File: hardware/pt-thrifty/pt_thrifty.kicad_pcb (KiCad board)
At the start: 2 copper layers, 25.4 x 31.6 mm, 23 parts, among them J1 Conn_01x09, J2 Conn_01x09, J3 SJ-43514-SMT-TR, SW1 PTS636 SM50J SMTR LFS, SW2 SW_Push_Shielded, U2 MCP6273T-E/CH

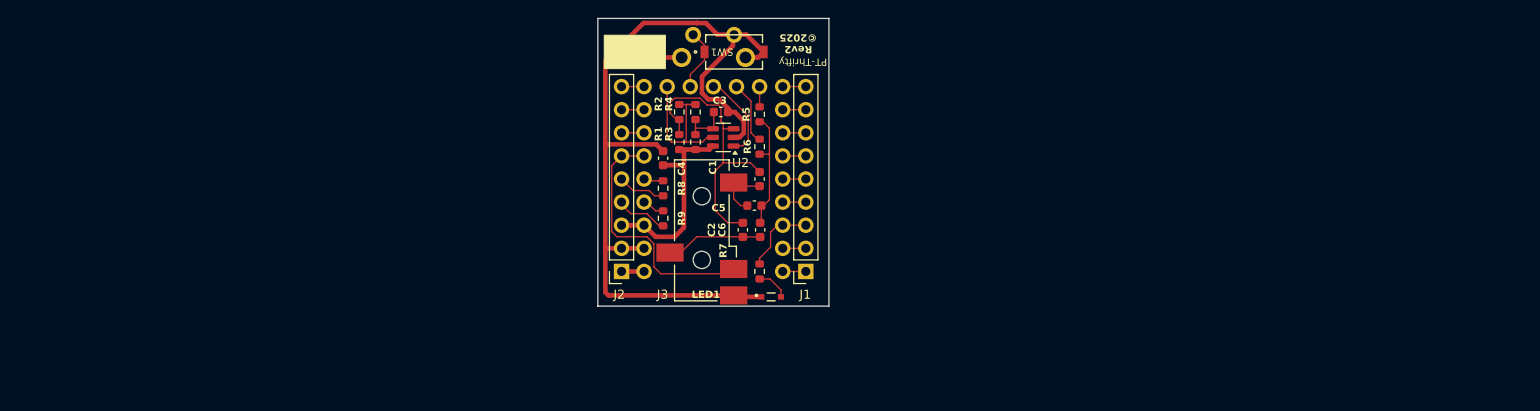
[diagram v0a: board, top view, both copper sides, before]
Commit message: WIP pt-thrifty rev3 sch/pcb
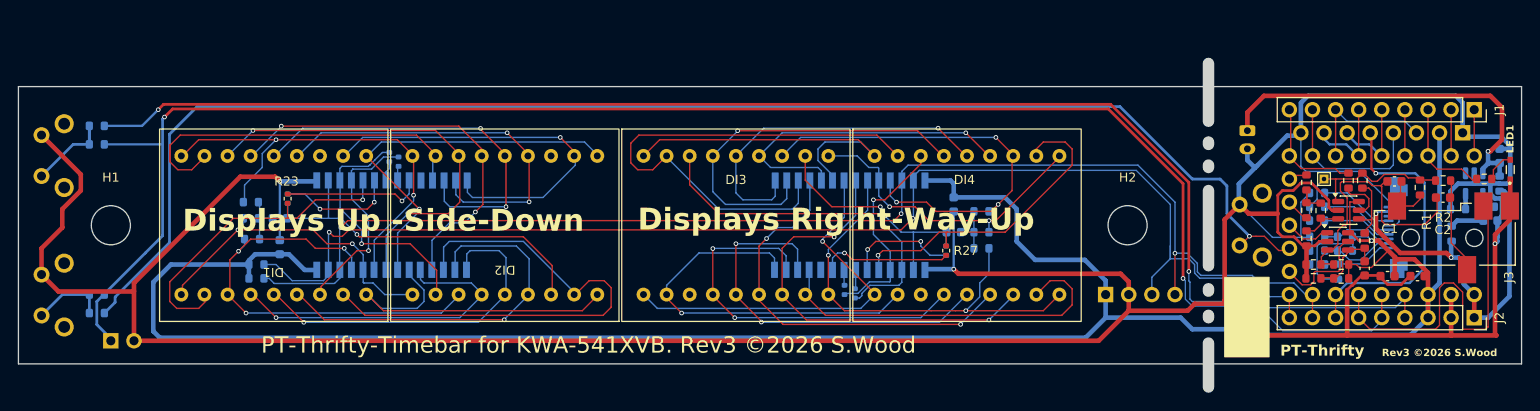
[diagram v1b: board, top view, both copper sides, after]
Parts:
- removed C6: 100nF, Capacitor_SMD:C_0603_1608Metric
- added C7: 10uF, Capacitor_SMD:C_0603_1608Metric, B.Cu at (166.3, 89.2)
- added C8: 10uF, Capacitor_SMD:C_0603_1608Metric, B.Cu at (92.2, 93.9)
- added C81: 1uF, Capacitor_SMD:C_0603_1608Metric, B.Cu at (225.3, 90.9)
- added C82: 1uF, Capacitor_SMD:C_0603_1608Metric, B.Cu at (226.3, 83.8)
- added D1: D, Diode_SMD:D_0603_1608Metric, B.Cu at (166.3, 92.2)
- added D2: D, Diode_SMD:D_0603_1608Metric, B.Cu at (92.2, 90.7)
- added DI1: KWA-541XVB, Displays:KWA-541XVB, F.Cu at (91.6, 91.4)
- added DI2: KWA-541XVB, Displays:KWA-541XVB, F.Cu at (117.0, 91.4)
- added DI3: KWA-541XVB, Displays:KWA-541XVB, F.Cu at (142.4, 91.4)
- added DI4: KWA-541XVB, Displays:KWA-541XVB, F.Cu at (167.8, 91.4)
- added H1: MountingHole, MountingHole:MountingHole_4.3mm_M4, F.Cu at (73.7, 91.4)
- added H2: MountingHole, MountingHole:MountingHole_4.3mm_M4, F.Cu at (185.4, 91.4)
- added J4: Conn_01x08, Connector_PinSocket_2.54mm:PinSocket_1x08_P2.54mm_Vertical, B.Cu at (222.2, 81.3)
- added J5: Conn_01x04, Connector_PinSocket_2.54mm:PinSocket_1x04_P2.54mm_Vertical, B.Cu at (183.0, 99.1)
- added J6: Conn_01x02, Connector_PinSocket_2.54mm:PinSocket_1x02_P2.54mm_Vertical, B.Cu at (73.7, 104.1)
- added J81: Conn_01x02, Connector_JST:JST_PH_B2B-PH-K_1x02_P2.00mm_Vertical, B.Cu at (198.6, 81.0)
- added J99: Conn_01x10, Connector_FFC-FPC:Amphenol_F32Q-1A7x1-11010_1x10-1MP_P0.5mm_Horizontal, B.Cu at (217.0, 91.7)
- added R10: 100K, Resistor_SMD:R_0603_1608Metric, F.Cu at (206.7, 89.8)
- added R11: 100K, Resistor_SMD:R_0603_1608Metric, F.Cu at (205.1, 92.9)
- added R12: 100K, Resistor_SMD:R_0603_1608Metric, F.Cu at (211.5, 93.1)
- added R13: 100K, Resistor_SMD:R_0603_1608Metric, F.Cu at (211.2, 86.5)
- added R14: 100R, Resistor_SMD:R_0603_1608Metric, F.Cu at (209.7, 86.5)
- added R15: 0R, Resistor_SMD:R_0603_1608Metric, B.Cu at (72.1, 101.1)
- added R16: 0R, Resistor_SMD:R_0603_1608Metric, B.Cu at (72.1, 99.1)
- added R17: 0R, Resistor_SMD:R_0603_1608Metric, B.Cu at (72.1, 80.5)
- added R18: 0R, Resistor_SMD:R_0603_1608Metric, B.Cu at (72.1, 82.5)
- added R20: 0R, Resistor_SMD:R_0402_1005Metric, B.Cu at (93.1, 88.5)
- added R21: 0R, Resistor_SMD:R_0402_1005Metric, B.Cu at (104.3, 83.9)
- added R22: 0R, Resistor_SMD:R_0402_1005Metric, B.Cu at (105.3, 84.5)
- added R23: 0R, Resistor_SMD:R_0402_1005Metric, F.Cu at (93.1, 88.5)
- added R24: 0R, Resistor_SMD:R_0402_1005Metric, B.Cu at (165.5, 94.2)
- added R25: 0R, Resistor_SMD:R_0402_1005Metric, B.Cu at (155.4, 98.9)
- added R26: 0R, Resistor_SMD:R_0402_1005Metric, B.Cu at (154.3, 98.6)
- added R27: 0R, Resistor_SMD:R_0402_1005Metric, F.Cu at (165.5, 94.2)
- added R28: 10K, Resistor_SMD:R_0603_1608Metric, B.Cu at (89.7, 95.8)
- added R29: 10K, Resistor_SMD:R_0603_1608Metric, B.Cu at (89.7, 97.3)
- added R30: 47K, Resistor_SMD:R_0603_1608Metric, B.Cu at (169.4, 89.9)
- added R31: 47K, Resistor_SMD:R_0603_1608Metric, B.Cu at (169.4, 92.2)
- added R32: 47K, Resistor_SMD:R_0603_1608Metric, B.Cu at (169.4, 94.0)
- added R33: 47K, Resistor_SMD:R_0603_1608Metric, B.Cu at (89.2, 93.0)
- added R34: 47K, Resistor_SMD:R_0603_1608Metric, B.Cu at (89.1, 90.7)
- added R35: 47K, Resistor_SMD:R_0603_1608Metric, B.Cu at (89.1, 88.9)
- added R81: 2.00K-1%, Resistor_SMD:R_0603_1608Metric, B.Cu at (221.7, 89.7)
- added R82: 100R, Resistor_SMD:R_0603_1608Metric, B.Cu at (226.6, 89.4)
- added R83: 100R, Resistor_SMD:R_0603_1608Metric, B.Cu at (221.0, 92.4)
- added R84: 100R, Resistor_SMD:R_0603_1608Metric, B.Cu at (226.3, 86.9)
- added R90: 100R, Resistor_SMD:R_0603_1608Metric, B.Cu at (222.4, 96.4)
- added R91: 100K, Resistor_SMD:R_0603_1608Metric, B.Cu at (208.5, 96.5)
- added R92: 100K, Resistor_SMD:R_0603_1608Metric, B.Cu at (206.3, 95.8)
- added R93: 100K, Resistor_SMD:R_0603_1608Metric, B.Cu at (209.3, 94.2)
- added R94: 100K, Resistor_SMD:R_0603_1608Metric, B.Cu at (206.3, 94.2)
- added R95: 100K, Resistor_SMD:R_0603_1608Metric, B.Cu at (209.3, 92.7)
- added R96: 100K, Resistor_SMD:R_0603_1608Metric, B.Cu at (206.3, 92.7)
- added R97: 100R, Resistor_SMD:R_0603_1608Metric, B.Cu at (206.2, 90.9)
- added R98: 100R, Resistor_SMD:R_0603_1608Metric, B.Cu at (206.2, 89.4)
- added R99: 100R, Resistor_SMD:R_0603_1608Metric, B.Cu at (206.2, 87.9)
- added SW3: SW_Push_Shielded, Button_Switch_THT:SW_Tactile_SPST_Angled_PTS645Vx31-2LFS, B.Cu at (66.0, 81.5)
- added TP1: TestPoint, TestPoint:TestPoint_THTPad_1.0x1.0mm_Drill0.5mm, F.Cu at (207.0, 86.4)
- added U3: MCP6273T, Package_TO_SOT_SMD:SOT-23-6, F.Cu at (209.7, 89.8)
- added U4: HT16K33A-28SSOP, HT9170D:SOIC28-1.27-11.5X17.5MM, B.Cu at (154.9, 91.4)
- added U5: HT16K33A-28SSOP, HT9170D:SOIC28-1.27-11.5X17.5MM, B.Cu at (104.5, 91.4)
- added U80: MCP73832-2-OT, Package_TO_SOT_SMD:SOT-23-5, B.Cu at (223.5, 86.9)
- C1, C2, C5: value 100nF -> 1uF
- R1, R2: value 10K -> 100R
- R3, R4: value 10K -> 100K
- R5: value 2.10K-1% -> 2.00K-1%
- R8: value 22R -> 2.00K-1%
- R9: value 22R -> 2.49K-1%
- SW1: value PTS636 SM50J SMTR LFS -> SW_Push_Shielded; footprint PicoTimecode_PCB_Rev2:SW_PTS636_CNK -> Button_Switch_THT:SW_Tactile_SPST_Angled_PTS645Vx31-2LFS; moved to B.Cu
- U2: value MCP6273T-E/CH -> MCP6273T
- moved U1 94.2 mm to (225.1, 100.4), turned to 90 degrees
- moved J2 93.9 mm to (223.5, 101.6), turned to -90 degrees
- moved J3 85.9 mm to (227.4, 89.3), turned to 180 degrees
- moved R2 84.3 mm to (220.1, 86.5), turned to 0 degrees
- moved LED1 82.4 mm to (227.5, 85.3), turned to 90 degrees
- moved R1 81.6 mm to (217.6, 87.3), turned to -90 degrees
- moved C4 80.7 mm to (214.0, 97.0), turned to 180 degrees
- moved SW2 80.6 mm to (66.0, 96.9), turned to -90 degrees
- moved R7 80.3 mm to (224.6, 86.4), turned to 0 degrees
- moved C2 77.0 mm to (220.1, 88.4), turned to 180 degrees
- moved J1 75.6 mm to (223.5, 78.7), turned to -90 degrees
- moved C5 73.3 mm to (217.3, 97.0)
- moved C3 72.8 mm to (211.5, 96.2), turned to -90 degrees
- moved R3 72.2 mm to (208.9, 95.8), turned to 180 degrees
- moved R8 70.7 mm to (205.1, 86.7)
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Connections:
- net Net-(J1-Pin_5) renamed /SPI0_DC
- net Net-(J1-Pin_6) renamed /SPI0_CSn
- net Net-(J1-Pin_7) renamed /SPI0_SCK
- net Net-(J1-Pin_8) renamed /SPI0_TX
- net Net-(J1-Pin_9) renamed /AMP_nEN1
- net Net-(J2-Pin_7) renamed /SPI0_RST
- net Net-(J2-Pin_8) renamed /I2C1_SCLK
- net Net-(J2-Pin_9) renamed /I2C1_SDA
- C5 pad 1: /IN_OUT_L -> GND
- C5 pad 2: Net-(C5-Pad2) -> +3.3V
- J2 pad 4: Net-(J2-Pin_4) -> /ROT_SW
- J2 pad 5: Net-(J2-Pin_5) -> /CLAP_SW
- R1 pad 1: +3.3V -> /OUTPUT
- R1 pad 2: /IN -> /IN_OUT_L
- R2 pad 1: /IN -> /OUTPUT
- R2 pad 2: /AMP_CS -> /IN_OUT_R
- R3 pad 2: /VREF -> /IN
- R4 pad 1: /VREF -> /IN
- R4 pad 2: /AMP_CS -> GND
- R5 pad 1: /LTC_TX -> +3.3V
- R5 pad 2: Net-(C5-Pad2) -> /VREF
- R6 pad 1: /nLTC_TX -> /VREF
- R6 pad 2: Net-(C5-Pad2) -> GND
- R8 pad 1: Net-(U1-GPIO28) -> /LTC_TX
- R8 pad 2: Net-(J2-Pin_5) -> Net-(R10-Pad1)
- R9 pad 1: Net-(U1-GPIO29) -> /nLTC_TX
- R9 pad 2: Net-(J2-Pin_4) -> Net-(R10-Pad1)
- SW1 pad 1: /KEYA -> GND
- SW1 pad 2: GND -> /KEYA
- SW2 pad 2: /KEYA -> Net-(R15-Pad2)
- U1 pad 14: Net-(U1-GPIO28) -> /CLAP_SW
- U1 pad 15: Net-(U1-GPIO29) -> /ROT_SW
- U1 pad 23: /AMP_CS -> /AMP_nEN0
- U2 pad 5: /AMP_CS -> /AMP_nEN0
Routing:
- net GND: track 101.3 -> 434.7 mm, vias 0 -> 3
- net +3.3V: track 23.4 -> 264.9 mm, vias 0 -> 1
- net /CLAP_SW: track 0.00 -> 189.8 mm, vias 0 -> 2
- net /ROT_SW: track 0.00 -> 164.4 mm, vias 0 -> 2
- net /KEYA: track 6.86 -> 157.1 mm, vias 0 -> 1
- net /I2C1_SCLK: track 2.48 -> 144.0 mm, vias 0 -> 3
- net /I2C1_SDA: track 2.48 -> 143.0 mm, vias 0 -> 2
- net /time-bar/HM_ROW8: track 0.00 -> 57.4 mm
- net /time-bar/SF_ROW8: track 0.00 -> 57.4 mm
- net /time-bar/HM_ROW2: track 0.00 -> 49.5 mm, vias 0 -> 2
- net /time-bar/HM_ROW0: track 0.00 -> 49.3 mm, vias 0 -> 3
- net /time-bar/SF_ROW2: track 0.00 -> 49.1 mm, vias 0 -> 2
- net /time-bar/SF_ROW0: track 0.00 -> 49.1 mm, vias 0 -> 3
- net /time-bar/SF_ROW3: track 0.00 -> 46.4 mm, vias 0 -> 2
- net /time-bar/HM_ROW3: track 0.00 -> 46.4 mm, vias 0 -> 2
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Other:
- board size 25.4 x 31.6 mm -> 165.2 x 35.6 mm
- board text added: "0"
- board text added: "0.0"
- board text added: "0.3"
- board text added: "0.4"
- board text added: "0.6"
- board text added: "0.65"
- board text added: "0.9"
- board text added: "1.2 inch"
- board text added: "16-Segment {dblquote}Time-Bar{dblquote} - for KWA-541XVB modules"
- board text added: "2026-07-28 © Simon Wood"
- board text added: "4.8"
- board text added: "5.2"
- board text added: "6.5 inch"
- board text added: "Displays Rig ht-Way-Up"
- board text added: "Displays Up -Side-Down"
- board text added: "PT Thrifty - lowest cost TimeCode"
- board text added: "PT-Thrifty-Timebar for KWA-541XVB. Rev3 ©2026 S.Wood"
- board text added: "Rev 3"
- board text added: "Rev3 ©2026 S.Wood"
- board text removed: "Rev2 ©2025"
